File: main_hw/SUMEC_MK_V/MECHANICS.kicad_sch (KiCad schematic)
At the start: 21 parts, among them SW2 SW_Push, SW3 SW_Push, SW4 SW_Push, SW5 SW_Push

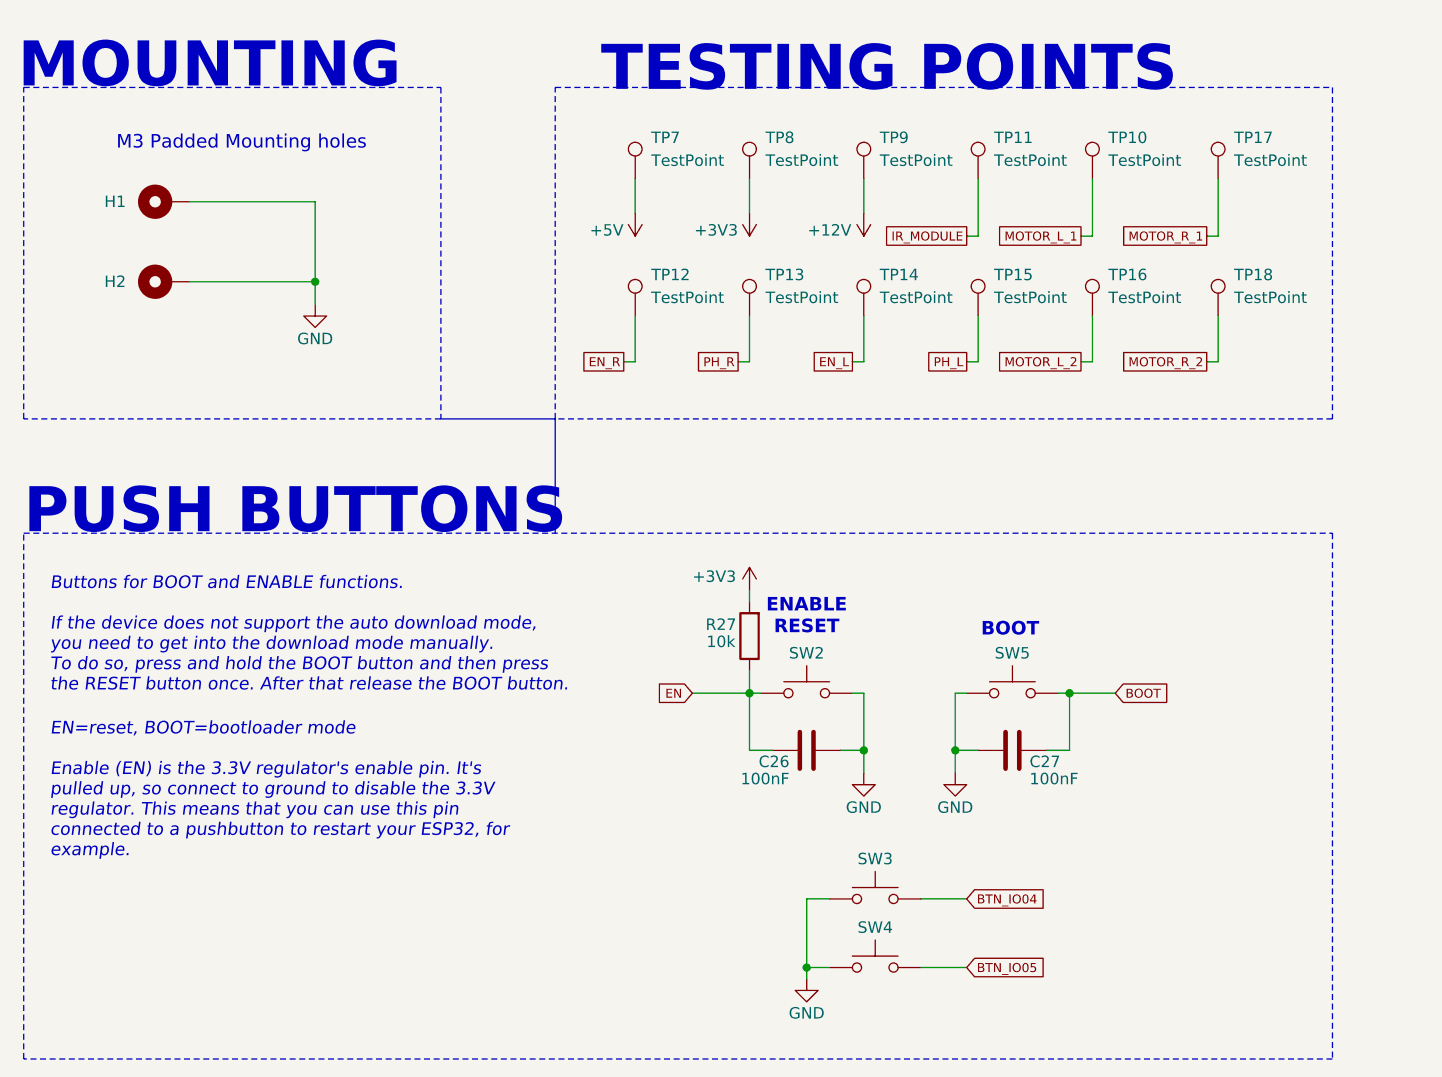
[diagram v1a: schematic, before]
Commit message: 67yfhtgftu
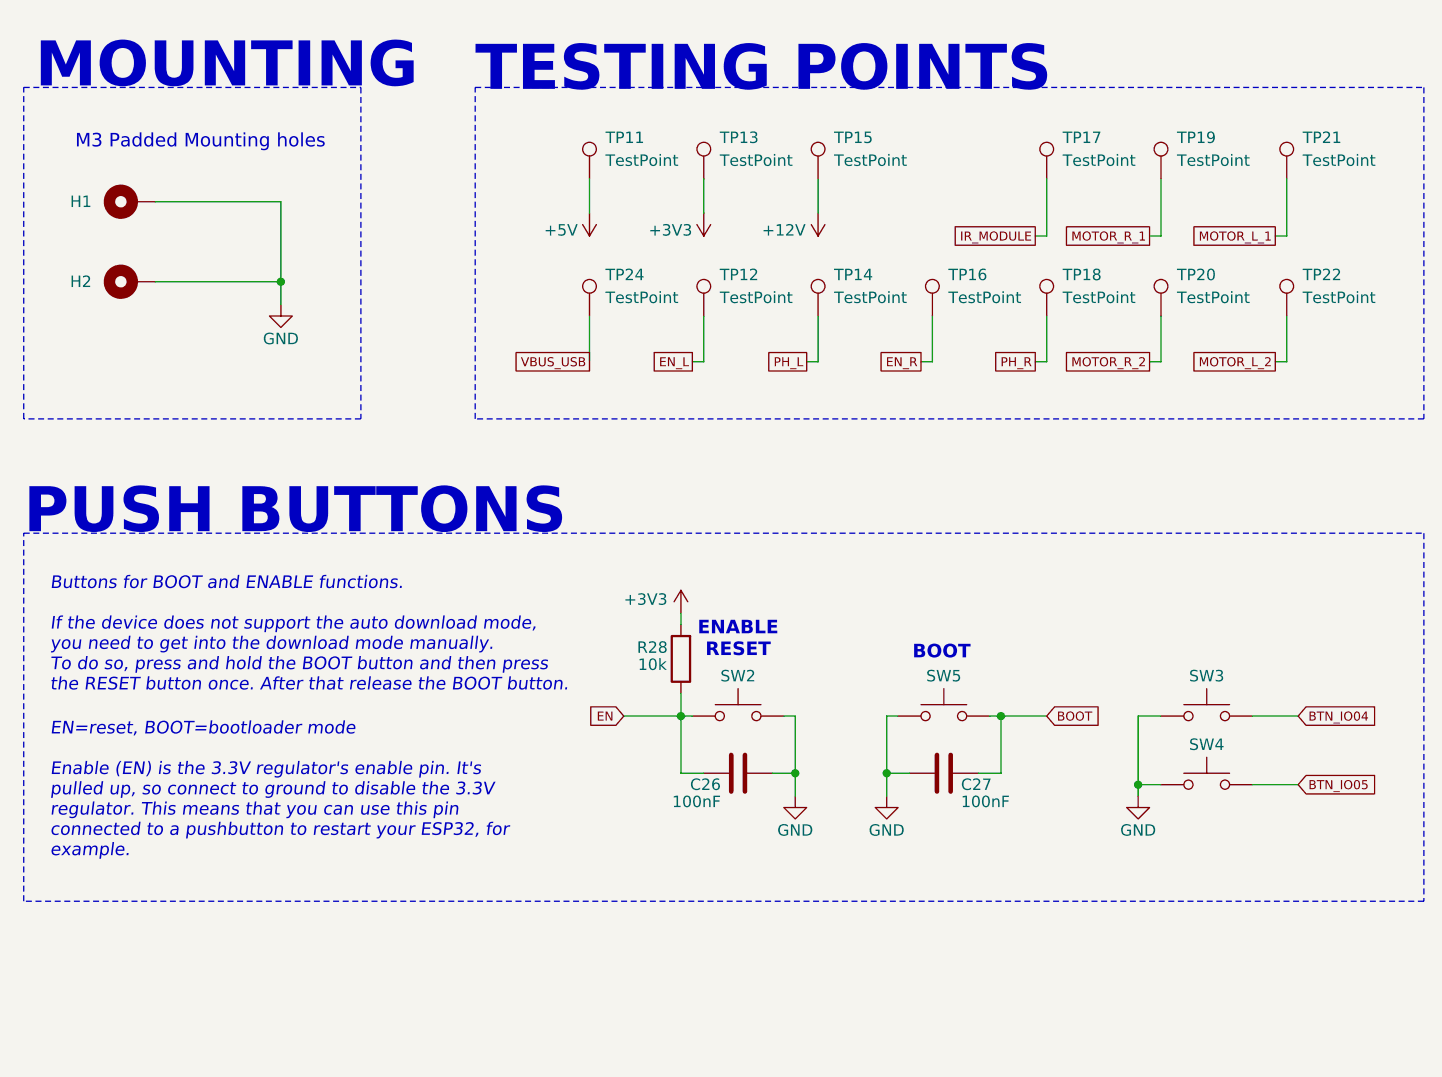
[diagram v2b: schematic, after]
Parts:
- added TP24: TestPoint, TestPoint:TestPoint_Pad_D1.0mm, symbol Connector:TestPoint
- renumbered R27 to R28, TP7 to TP11, TP8 to TP13, TP13 to TP14, TP9 to TP15, TP14 to TP16, TP11 to TP17, TP15 to TP18, TP10 to TP19, TP16 to TP20, TP17 to TP21, TP18 to TP22
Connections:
- net EN_L: now also TP12.1; no longer TP16.1
- net EN_R: now also TP16.1; no longer TP12.1
- net MOTOR_L_1: now also TP21.1; no longer TP19.1
- net MOTOR_L_2: now also TP22.1; no longer TP20.1
- net MOTOR_R_1: now also TP19.1; no longer TP21.1
- net MOTOR_R_2: now also TP20.1; no longer TP22.1
- net PH_L: now also TP14.1; no longer TP18.1
- net PH_R: now also TP18.1; no longer TP14.1
- new net VBUS_USB: TP24.1
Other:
- moved on the sheet: C26, C27, H1, H2, R28, SW2, SW3, SW4, SW5, TP11, TP12, TP13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
